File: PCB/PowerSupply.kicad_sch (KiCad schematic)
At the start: 22 parts, among them IC19 TPS54302DDCT, IC28 LM75BD,118, J20 Screw_Terminal_01x02

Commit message: Implementação do novo circuito do Wleding detector; correcao dos campos dos componentes
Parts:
- C104: Distribuidor Mouser -> (none); Link https://pt.mouser.com/ProductDetail/Samsung-Electro-Mechani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 -> (none); MPN (none) -> CL10B104MB8NNNC; Ref CL10B104MB8NNNC -> (none)
- C88: Field6 RM EMK105 B7104KV-F -> (none); Field7 TAIYO YUDEN EUROPE GMBH -> (none); Field8 110091611 -> (none); Mouser Link https://pt.mouser.com/ProductDetail/Samsung-Electro-Mechani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 -> (none); Mouser Part Number CL31B104KBCNNND -> (none); Part Description 0.1uF 10% 16V Ceramic Capacitor X7R 0402 (1005 Metric) -> (none)
- C89, C90, C91: Field4 Digikey -> (none); Field5 490-10505-1-ND -> (none); Field6 GRM21BC8YA106KE11L -> (none); Field7 Murata -> (none); Part Description 10uF 10% or 20% 35V Ceramic Capacitor X6S 0805 (2012 Metric) -> (none)
- IC19: Height 1.1 -> (none); Manufacturer_Name Texas Instruments -> (none); Manufacturer_Part_Number TPS54302DDCT -> (none); Mouser Part Number 595-TPS54302DDCT -> (none); Mouser Price/Stock https://www.mouser.co.uk/ProductDetail/Texas-Instruments/TP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 -> (none)
- IC28: Height 1.75 -> (none); Manufacturer_Name NXP -> (none); Manufacturer_Part_Number LM75BD,118 -> (none); Mouser Part Number 771-LM75BD118 -> (none); Mouser Price/Stock https://www.mouser.co.uk/ProductDetail/NXP-Semiconductors/L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 -> (none)
- L1: Height 3 -> (none); Manufacturer_Name Bourns -> (none); Manufacturer_Part_Number SRP7028CC-6R8M -> (none); Mouser Part Number 652-SRP7028CC-6R8M -> (none); Mouser Price/Stock https://www.mouser.co.uk/ProductDetail/Bourns/SRP7028CC-6R8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 -> (none)
- R111, R113, R51, R67: Field4 Farnell -> (none); Field5 9239278 -> (none); Field6 RK73G1ETQTP2201D -> (none); Field7 KOA EUROPE GMBH -> (none); Field8 120889581 -> (none); Part Description Resistor 2.2K M1005 1% 63mW -> (none)
- R144, R145, R146: Distribuidor Mouser -> (none); Link https://pt.mouser.com/ProductDetail/Vishay-Draloric/RCS0603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 -> (none); MPN (none) -> RCS060310K0FKEA; Ref RCS060310K0FKEA -> (none)
- R147, R148: Distribuidor Mouser -> (none); Link https://pt.mouser.com/ProductDetail/YAGEO/RE0603FRE07150RL?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 -> (none); MPN (none) -> RE0603FRE07150RL; Ref RE0603FRE07150RL -> (none)

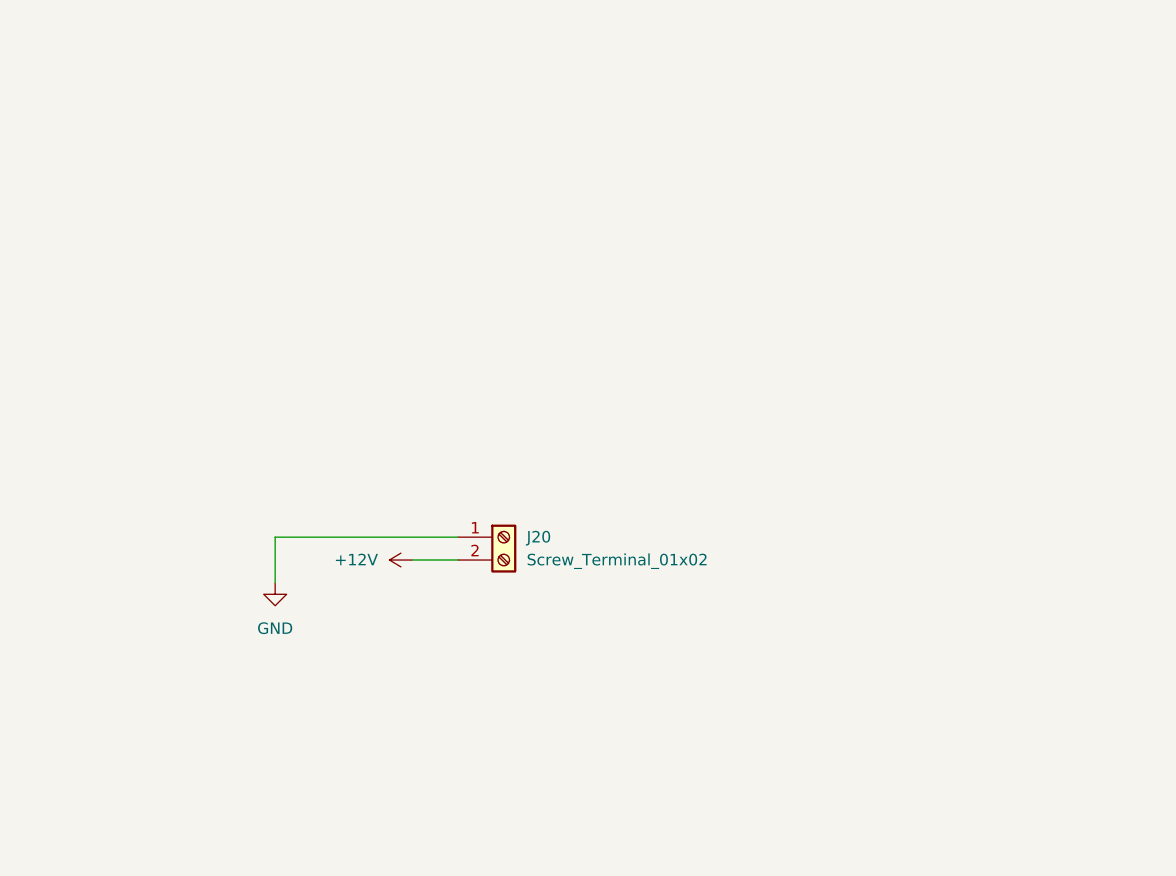
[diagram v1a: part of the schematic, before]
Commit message: Layout finalizado
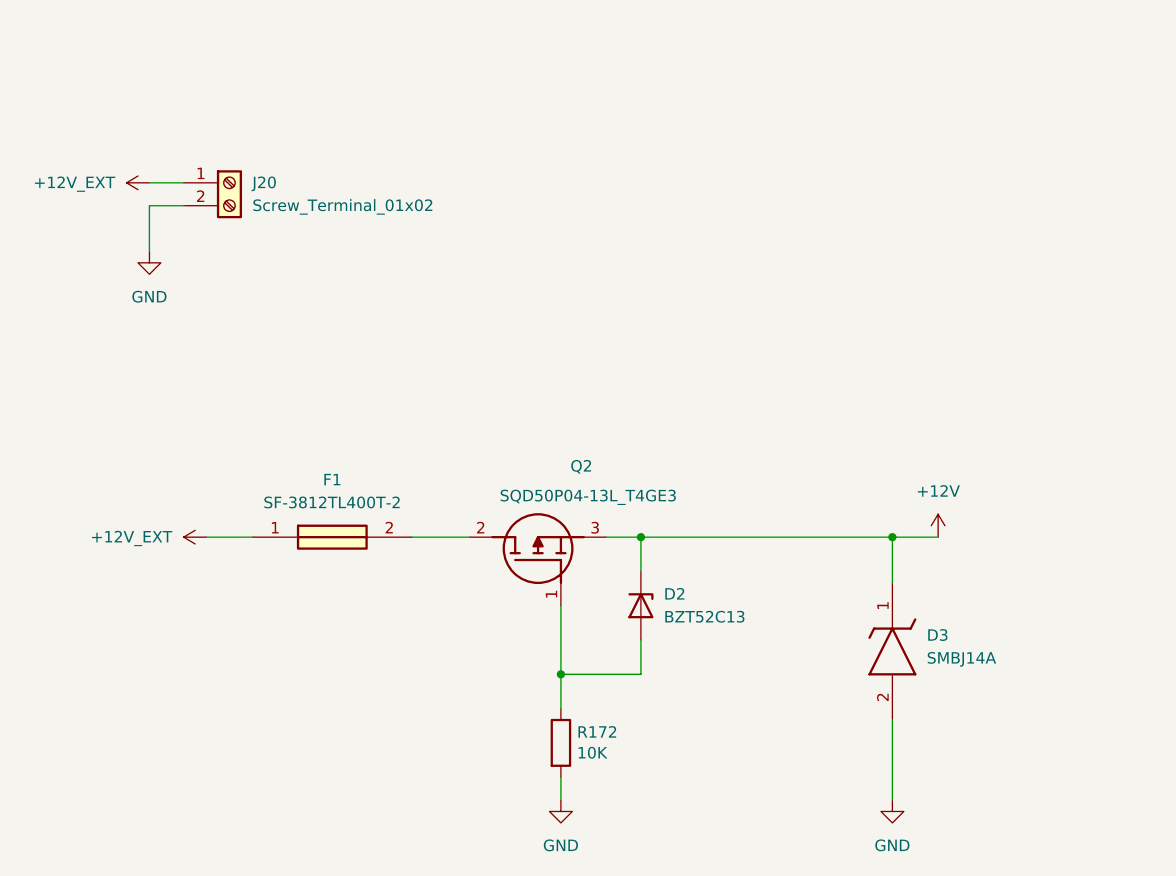
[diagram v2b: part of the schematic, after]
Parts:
- added D2: BZT52C13, Diode_SMD:D_SOD-123, symbol Diode:BZT52Bxx
- added D3: SMBJ14A, FOOTPRINTS:DIOM5436X261N, symbol SMBJ15A:SMBJ15A
- added F1: SF-3812TL400T-2, FOOTPRINTS:SF3812TL400T2, symbol SF-3812TL400T-2:SF-3812TL400T-2
- added Q2: SQD50P04-13L_T4GE3, FOOTPRINTS:SQD50P0413L_T4GE3, symbol SQD50P04-13L_T4GE3:SQD50P04-13L_T4GE3
- added R172: 10K, Resistor_SMD:R_0603_1608Metric, symbol Device:R
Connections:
- net +12V: now also D2.1 (K), D3.1 (K), Q2.3 (S); no longer J20.2 (Pin_2)
- net GND: now also J20.2 (Pin_2), D3.2 (A), R172.2; no longer J20.1 (Pin_1)
- new net: F1.2, Q2.2 (D)
- new net: D2.2 (A), Q2.1 (G), R172.1
- new net +12V_EXT: F1.1, J20.1 (Pin_1)
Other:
- moved on the sheet: J20
